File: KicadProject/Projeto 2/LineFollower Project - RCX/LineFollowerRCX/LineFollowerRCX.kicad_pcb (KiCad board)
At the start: 2 copper layers, 100 x 70.9 mm, 13 parts, among them J1 Conn_01x11_Pin, J10 GND pinos, J2 Motor 1, J3 Motor 1, J4 Modulo bluetooth, J7 Conector sensor lateral Esque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, J8 Conector sensor lateral Direi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, J9 VCC pinos, U1 ROB-14450, U2 LM7805_TO220

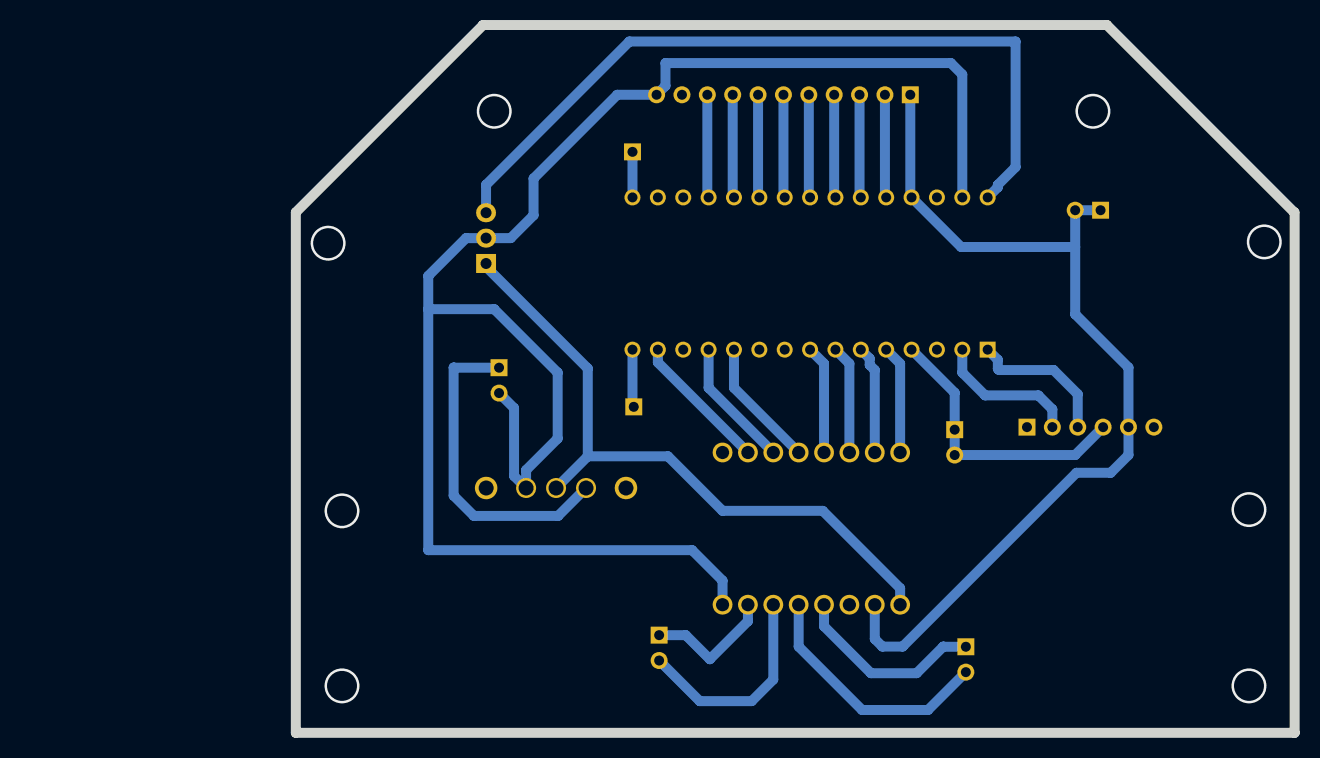
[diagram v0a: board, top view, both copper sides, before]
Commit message: Infelizmente não foi :(
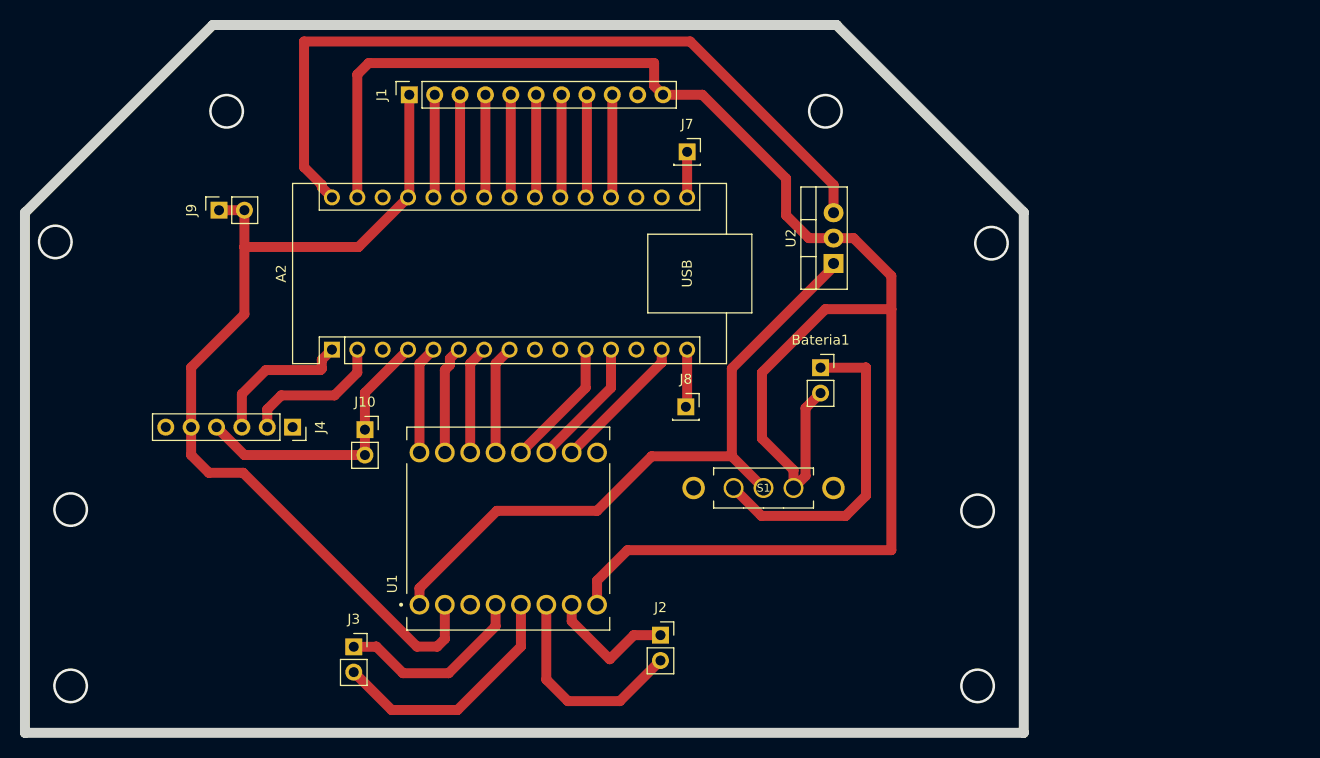
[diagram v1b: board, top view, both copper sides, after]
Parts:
- A2, Bateria1, J1, J10, J2, J3, J4, J7, J8, J9, S1, U1, U2: moved to F.Cu
- moved J9 88.3 mm to (130.8, 102.7)
- moved J4 73.5 mm to (138.2, 124.5)
- moved A2 65.7 mm to (142.1, 116.7)
- moved J3 61.3 mm to (144.3, 146.5), turned to 0 degrees
- moved J10 59.0 mm to (145.4, 124.7), turned to 0 degrees
- moved J1 50.2 mm to (149.9, 91.2)
- moved U2 34.8 mm to (192.3, 108.1)
- moved Bateria1 32.2 mm to (191.0, 118.5), turned to 0 degrees
- moved U1 30.3 mm to (159.8, 134.6)
- moved S1 20.8 mm to (185.3, 130.6), turned to 0 degrees
- moved J7 5.47 mm to (177.7, 96.9), turned to 0 degrees
- moved J8 5.22 mm to (177.5, 122.4), turned to 0 degrees
- moved J2 0.14 mm to (175.0, 145.3), turned to 0 degrees
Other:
- outline, holes or cut-outs redrawn
